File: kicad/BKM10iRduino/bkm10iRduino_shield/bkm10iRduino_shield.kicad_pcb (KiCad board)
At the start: 4 copper layers, 20.3 x 80 mm, 6 parts, among them J1 RJ45, SW1 SW_SPST, U1 TSOP343xx, U2 MAX485E

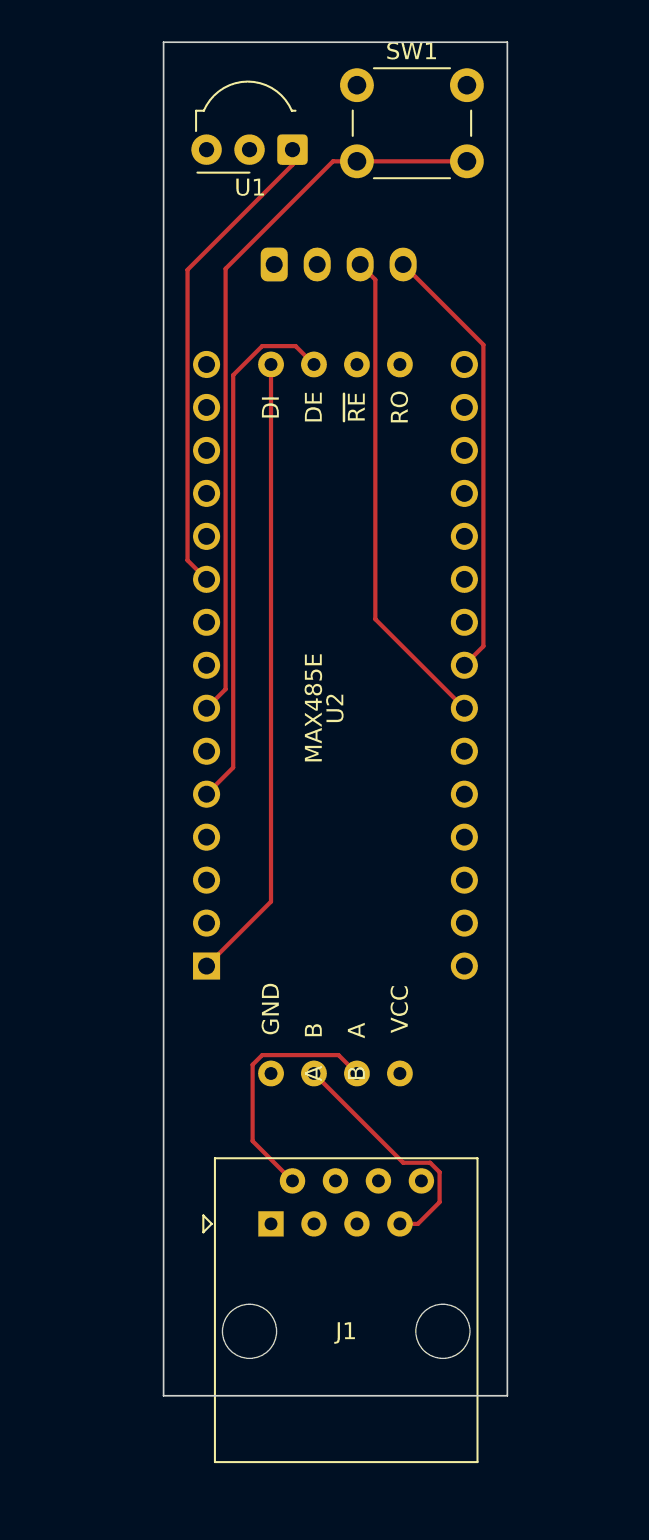
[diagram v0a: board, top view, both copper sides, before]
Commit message: updated pcb design
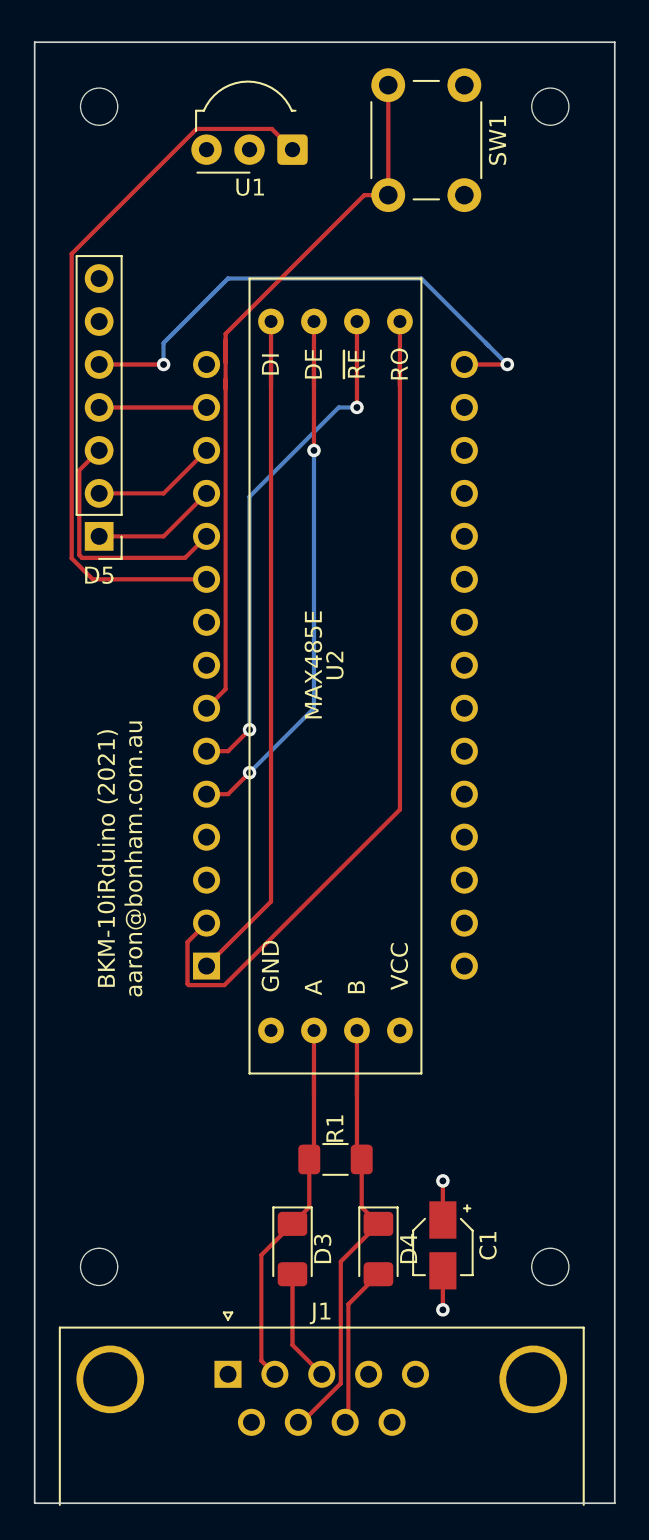
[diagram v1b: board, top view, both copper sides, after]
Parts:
- removed Brd1: SSD1306, SSD1306:128x64OLED
- added C1: C_Small, Capacitor_SMD:CP_Elec_3x5.3, F.Cu at (174.0, 120.7)
- added D3: D_Small_ALT, Diode_SMD:D_1206_3216Metric_Pad1.42x1.75mm_HandSolder, F.Cu at (165.1, 120.9)
- added D4: D_Small_ALT, Diode_SMD:D_1206_3216Metric_Pad1.42x1.75mm_HandSolder, F.Cu at (170.2, 120.9)
- added D5: SH1106, Connector_PinHeader_2.54mm:PinHeader_1x07_P2.54mm_Vertical, F.Cu at (153.7, 78.7)
- added R1: R, Resistor_SMD:R_1206_3216Metric_Pad1.30x1.75mm_HandSolder, F.Cu at (167.6, 115.6)
- added REF**: MountingHole_2.2mm_M2, MountingHole:MountingHole_2.2mm_M2, F.Cu at (180.3, 121.9)
- added REF**: MountingHole_2.2mm_M2, MountingHole:MountingHole_2.2mm_M2, F.Cu at (153.7, 121.9)
- added REF**: MountingHole_2.2mm_M2, MountingHole:MountingHole_2.2mm_M2, F.Cu at (180.3, 53.3)
- added REF**: MountingHole_2.2mm_M2, MountingHole:MountingHole_2.2mm_M2, F.Cu at (153.7, 53.3)
- A1: footprint Module:Arduino_Nano -> bkm10rduino:Arduino_Nano
- J1: value RJ45 -> DB9_Male; footprint Connector_RJ:RJ45_Amphenol_54602-x08_Horizontal -> Connector_Dsub:DSUB-9_Male_Horizontal_P2.77x2.84mm_EdgePinOffset4.94mm_Housed_MountingHolesOffset7.48mm
- moved J1 9.25 mm to (161.3, 128.3)
- moved SW1 6.35 mm to (175.3, 52.1), turned to 270 degrees
- moved U2 2.54 mm to (171.4, 108.0)
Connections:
- net Net-(J1-Pad2) renamed AB+
- net Net-(J1-Pad7) renamed AB-
- net ~LEARN_BUTTON_IN renamed LEARN_BUTTON_IN
- A1 pad 11: Net-(A1-Pad11) -> RES
- A1 pad 12: Net-(A1-Pad12) -> CS
- A1 pad 13: Net-(A1-Pad13) -> DC
- A1 pad 14: Net-(A1-Pad14) -> MOSI
- A1 pad 16: Net-(A1-Pad16) -> SCK
- A1 pad 2: Net-(A1-Pad2) -> RS485_RX
- A1 pad 6: Net-(A1-Pad6) -> RS485_RX_ENABLE
- J1 pad 3: Net-(J1-Pad3) -> YZ+
- J1 pad 8: Net-(J1-Pad8) -> YZ-
- U2 pad 1: Net-(U2-Pad1) -> RS485_RX
- U2 pad 2: Net-(U2-Pad2) -> RS485_RX_ENABLE
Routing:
- net RS485_RX: track 0.00 -> 51.1 mm
- net SCK: track 0.00 -> 31.9 mm, vias 0 -> 2
- net RS485_RX_ENABLE: track 0.00 -> 30.5 mm, vias 0 -> 2
- net Net-(A1-Pad24): track 28.8 -> 0.00 mm
- net Net-(A1-Pad23): track 26.1 -> 0.00 mm
- net RES: track 0.00 -> 14.8 mm
- net IR_OUT: track 28.4 -> 43.1 mm
- net AB-: track 14.5 -> 27.0 mm
- net YZ-: track 0.00 -> 9.57 mm
- net AB+: track 14.7 -> 23.2 mm
- net DC: track 0.00 -> 7.40 mm
- net CS: track 0.00 -> 7.40 mm
- net YZ+: track 0.00 -> 6.63 mm
- net MOSI: track 0.00 -> 6.35 mm
- net RS485_TX: track 37.1 -> 40.9 mm
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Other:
- board size 20.3 x 80 mm -> 34.3 x 86.4 mm
- board text added: "Arduino Nano"
- board text added: "BKM-10iRduino (2021) aaron@bonham.com.au"
- board text added: "CK"
- board text added: "CS"
- board text added: "DC"
- board text added: "GND"
- board text added: "MOSI"
- board text added: "RES"
- board text added: "VCC"
- board text removed: "A"
- board text removed: "B"
